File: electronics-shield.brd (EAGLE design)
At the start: 85 x 56 mm, 79 parts, among them IC1 TLE9201SG, IC2 TLE9201SG, IC3 TLE9201SG, IC4 TLE9201SG, IC5 LINEAR_MCP1703CB, J1 USB-MICRO-B, Q1 USER-SUBMITTED_MOSFET-PCHANNE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, Q2 ON-SEMICONDUCTOR---NTZD3154NT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, Q3 ON-SEMICONDUCTOR---NTZD3154NT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, U1 STM32F0XX8T, U2 EEPROM-I2C, X1 CONNECTOR_PHOENIX_3.81, X2 Listwa zaciskowa rozłączalna 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, Y1 8 MHz

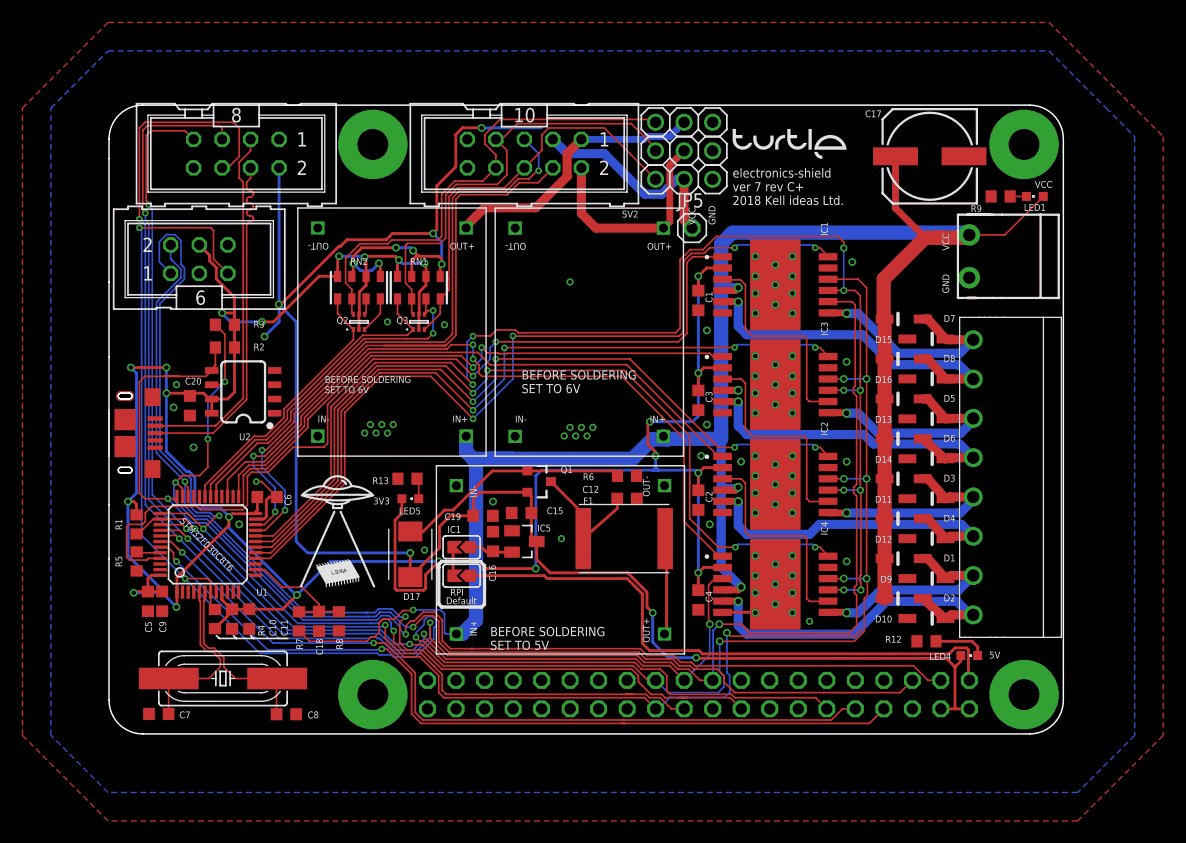
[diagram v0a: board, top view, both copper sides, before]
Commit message: 7C+ release
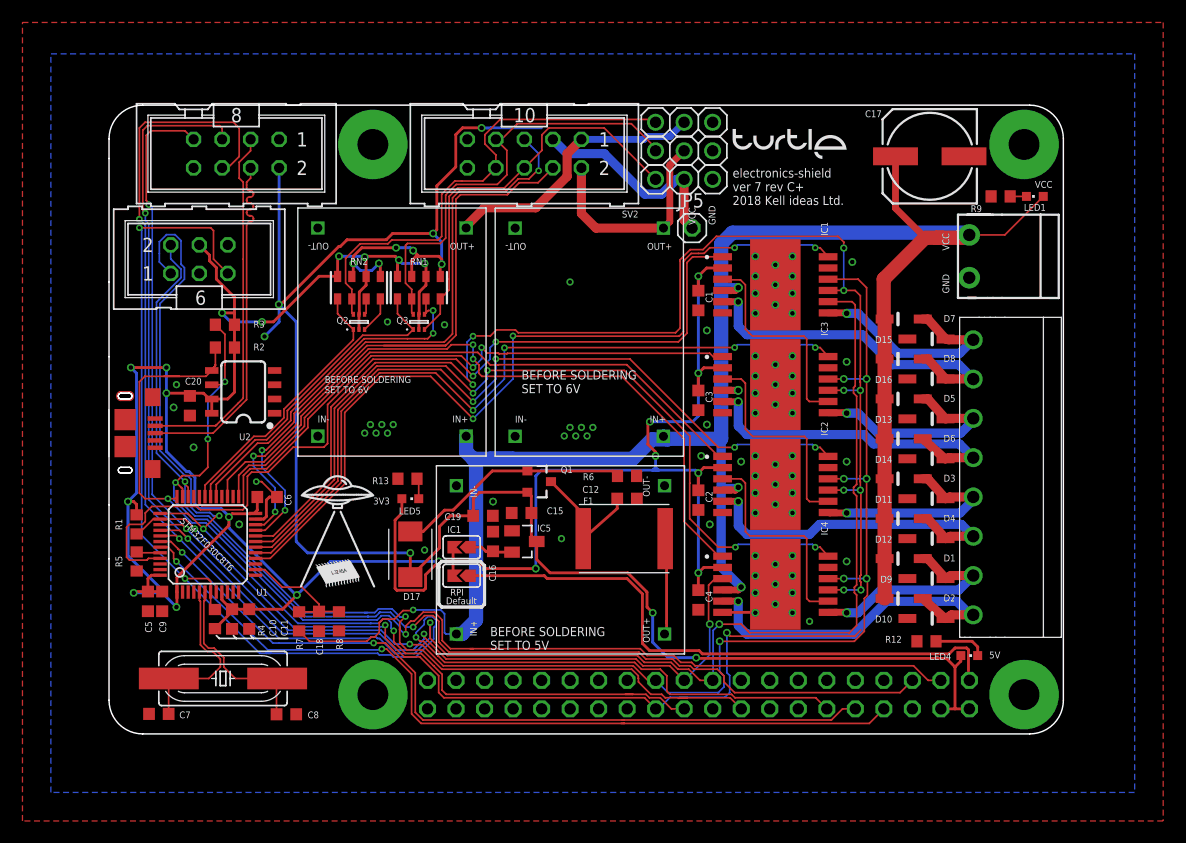
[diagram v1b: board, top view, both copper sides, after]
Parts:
- JP5: value (none) -> Listwa kołkowa 2.54mm prosta 1x1 (1pin)
- Q2, Q3: value ON-SEMICONDUCTOR---NTZD3154NT1G_ON_SEMICONDUCTOR_NTZD3154NT1GON_SEMICONDUCTOR_NTZD3154NT1G_0_0 -> NTZD3154NT1G
- SV1: value gniazdo IDC męskie 6pin proste -> Gniazdo IDC męskie 6pin proste
- SV2: value (none) -> Gniazdo IDC męskie 10pin proste
- SV3: value ML8 -> Gniazdo IDC męskie 8pin proste
- renumbered $3_0_$_2018-08-14_21-12-08 to IC6, $3_1_$_2018-08-14_21-12-08 to IC7, $3_2_$_2018-08-14_21-12-08 to IC8
